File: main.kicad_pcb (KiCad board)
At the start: 2 copper layers, 241.2 x 99.3 mm, 99 parts, among them SW1 Kailh-Choc, SW10 Kailh-Choc, SW11 Kailh-Choc, SW12 Kailh-Choc, SW13 Kailh-Choc, SW14 Kailh-Choc, SW15 Kailh-Choc, SW16 Kailh-Choc, SW17 Kailh-Choc, SW18 Kailh-Choc, SW19 Kailh-Choc, SW2 Kailh-Choc, SW20 Kailh-Choc, SW21 Kailh-Choc, SW22 Kailh-Choc, SW23 Kailh-Choc, SW24 Kailh-Choc, SW25 Kailh-Choc, SW26 Kailh-Choc, SW27 Kailh-Choc, SW28 Kailh-Choc, SW29 Kailh-Choc, SW3 Kailh-Choc, SW30 Kailh-Choc, SW31 Kailh-Choc, SW32 Kailh-Choc, SW33 Kailh-Choc, SW34 Kailh-Choc, SW4 Kailh-Choc, SW5 Kailh-Choc, SW6 Kailh-Choc, SW7 Kailh-Choc, SW8 Kailh-Choc, SW9 Kailh-Choc, U1 nice_nano, U2 nice_nano

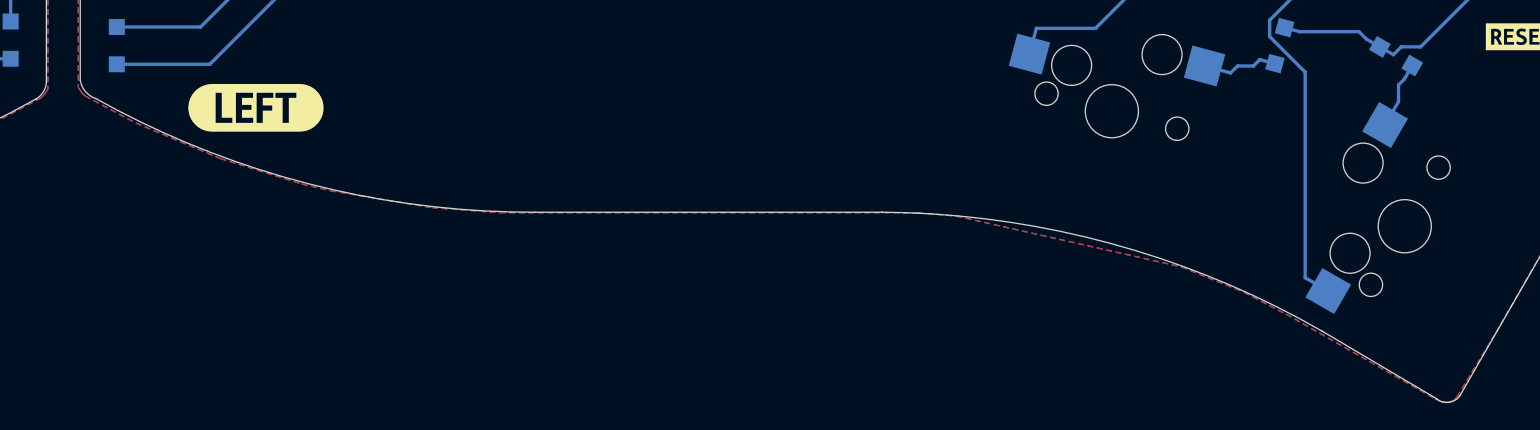
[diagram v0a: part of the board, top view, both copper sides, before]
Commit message: minor update to PCB and name changes
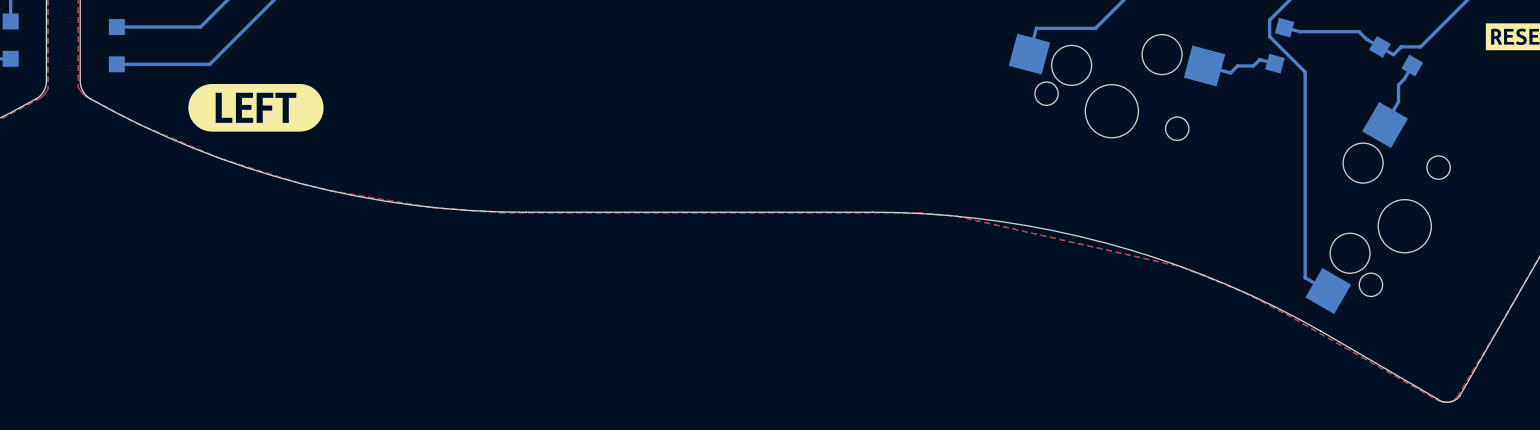
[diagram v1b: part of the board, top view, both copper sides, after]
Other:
- outline, holes or cut-outs redrawn
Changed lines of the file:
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@@
   (paper "A4")
   (title_block
-    (title "Urchin on Steroids")
+    (title "Ursa - Urchin on Steroids")
     (rev "v.1.0")
   )
@@
       (sketchpadsonfab false)
       (subtractmaskfromsilk false)
-      (outputformat 1)
+      (outputformat 5)
       (mirror false)
-      (drillshape 1)
+      (drillshape 0)
       (scaleselection 1)
       (outputdirectory "")
@@
   (gr_line (start 148.860169 106.299) (end 148.463 106.299) (layer "Edge.Cuts") (width 0.05))
   (gr_line (start 148.860169 106.299) (end 148.860169 120.866113) (layer "Edge.Cuts") (width 0.05))
+  (gr_line (start 252.431036 144.572711) (end 265.176 122.428) (layer "Edge.Cuts") (width 0.05))
   (gr_line (start 146.304 63.881) (end 146.304 83.680513) (layer "Edge.Cuts") (width 0.05))
   (gr_arc (start 146.320169 120.866113) (mid 146.131261 121.669384) (end 145.558169 122.263113) (layer "Edge.Cuts") (width 0.05))
   (gr_arc (start 145.558169 122.263113) (mid 129.751355 128.625656) (end 112.847803 130.772113) (layer "Edge.Cuts") (width 0.05))
   (gr_arc (start 249.047 70.542191) (mid 248.101986 70.229033) (end 247.65 69.342) (layer "Edge.Cuts") (width 0.05))
+  (gr_arc (start 182.332535 130.772113) (mid 165.428983 128.625656) (end 149.622169 122.263113) (layer "Edge.Cuts") (width 0.05))
   (gr_arc (start 148.463 101.219) (mid 147.574 101.808697) (end 146.685 101.219) (layer "Edge.Cuts") (width 0.05))
   (gr_line (start 146.304 101.219) (end 146.685 101.219) (layer "Edge.Cuts") (width 0.05))
-  (gr_arc (start 209.059148 130.772113) (mid 226.154025 133.098935) (end 242.09375 139.7) (layer "Edge.Cuts") (width 0.05))
   (gr_line (start 53.18125 139.7) (end 44.45 144.78) (layer "Edge.Cuts") (width 0.05))
   (gr_line (start 47.573589 56.884499) (end 47.573589 69.469) (layer "Edge.Cuts") (width 0.05))
   (gr_line (start 146.320169 106.299) (end 146.685 106.299) (layer "Edge.Cuts") (width 0.05))
   (gr_arc (start 44.45 144.78) (mid 43.587846 144.96327) (end 42.8625 144.4625) (layer "Edge.Cuts") (width 0.05))
+  (gr_arc (start 208.338331 130.772113) (mid 225.746285 133.058428) (end 241.999088 139.7) (layer "Edge.Cuts") (width 0.05))
   (gr_arc (start 94.377169 45.809113) (mid 121.522294 49.731191) (end 145.669 62.738) (layer "Edge.Cuts") (width 0.05))
   (gr_arc (start 148.844 63.881) (mid 149.013525 63.227292) (end 149.479 62.738) (layer "Edge.Cuts") (width 0.05))
-  (gr_arc (start 183.053352 130.772113) (mid 165.986032 128.633745) (end 150.01875 122.2375) (layer "Edge.Cuts") (width 0.05))
   (gr_line (start 30.115169 122.390113) (end 42.8625 144.4625) (layer "Edge.Cuts") (width 0.05))
   (gr_arc (start 53.18125 139.7) (mid 69.434053 133.058427) (end 86.842007 130.772113) (layer "Edge.Cuts") (width 0.05))
@@
   (gr_line (start 148.844 63.881) (end 148.844 83.693) (layer "Edge.Cuts") (width 0.05))
   (gr_arc (start 47.573589 56.884499) (mid 47.693177 56.478417) (end 48.01359 56.201738) (layer "Edge.Cuts") (width 0.05))
+  (gr_arc (start 149.622169 122.263113) (mid 149.049068 121.669395) (end 148.860169 120.866113) (layer "Edge.Cuts") (width 0.05))
   (gr_arc (start 149.479 62.738) (mid 171.224146 50.176089) (end 195.961 45.847) (layer "Edge.Cuts") (width 0.05))
-  (gr_line (start 250.698 144.78) (end 242.09375 139.7) (layer "Edge.Cuts") (width 0.05))
-  (gr_line (start 252.431036 144.572711) (end 265.176 122.428) (layer "Edge.Cuts") (width 0.05))
   (gr_arc (start 146.685 106.299) (mid 147.574 105.705003) (end 148.463 106.299) (layer "Edge.Cuts") (width 0.05))
   (gr_line (start 112.847803 130.772113) (end 86.842007 130.772113) (layer "Edge.Cuts") (width 0.05))
   (gr_line (start 27.432 70.485) (end 46.228 70.485) (layer "Edge.Cuts") (width 0.05))
-  (gr_line (start 209.059148 130.772113) (end 183.053352 130.772113) (layer "Edge.Cuts") (width 0.05))
   (gr_arc (start 195.961 45.847) (mid 222.113777 48.419233) (end 247.202529 56.238357) (layer "Edge.Cuts") (width 0.05))
-  (gr_arc (start 252.431036 144.572711) (mid 251.609177 145.04973) (end 250.698 144.78) (layer "Edge.Cuts") (width 0.05))
+  (gr_line (start 208.338331 130.772113) (end 182.332535 130.772113) (layer "Edge.Cuts") (width 0.05))
   (gr_line (start 268.223874 70.993) (end 268.224127 108.204) (layer "Edge.Cuts") (width 0.05))
+  (gr_line (start 250.730338 144.78) (end 241.999088 139.7) (layer "Edge.Cuts") (width 0.05))
   (gr_arc (start 267.589 70.485) (mid 268.011647 70.607513) (end 268.223874 70.993) (layer "Edge.Cuts") (width 0.05))
   (gr_arc (start 146.685 88.773) (mid 147.574 88.184548) (end 148.463 88.773) (layer "Edge.Cuts") (width 0.05))
+  (gr_arc (start 252.431036 144.572711) (mid 251.625346 145.042759) (end 250.730338 144.78) (layer "Edge.Cuts") (width 0.05))
   (gr_line (start 146.320169 120.866113) (end 146.320169 106.299) (layer "Edge.Cuts") (width 0.05))
   (gr_arc (start 27.051 70.866) (mid 27.162592 70.596592) (end 27.432 70.485) (layer "Edge.Cuts") (width 0.05))
   (gr_arc (start 148.463 83.693) (mid 147.569848 84.277833) (end 146.685 83.680513) (layer "Edge.Cuts") (width 0.05))
   (gr_arc (start 47.573589 69.469) (mid 47.109483 70.253367) (end 46.228 70.485) (layer "Edge.Cuts") (width 0.05))
-  (gr_arc (start 150.01875 122.2375) (mid 149.250894 121.711111) (end 148.860169 120.866113) (layer "Edge.Cuts") (width 0.05))
   (gr_line (start 148.844 88.773) (end 148.463 88.773) (layer "Edge.Cuts") (width 0.05))
   (gr_line (start 247.65 69.342) (end 247.65 56.896) (layer "Edge.Cuts") (width 0.05))
